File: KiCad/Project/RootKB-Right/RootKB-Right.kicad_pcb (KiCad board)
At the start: 2 copper layers, 137.4 x 107.4 mm, 69 parts, among them J1 OLED-128x32, U1 Arduino_Pro_Micro, U2 TRRS

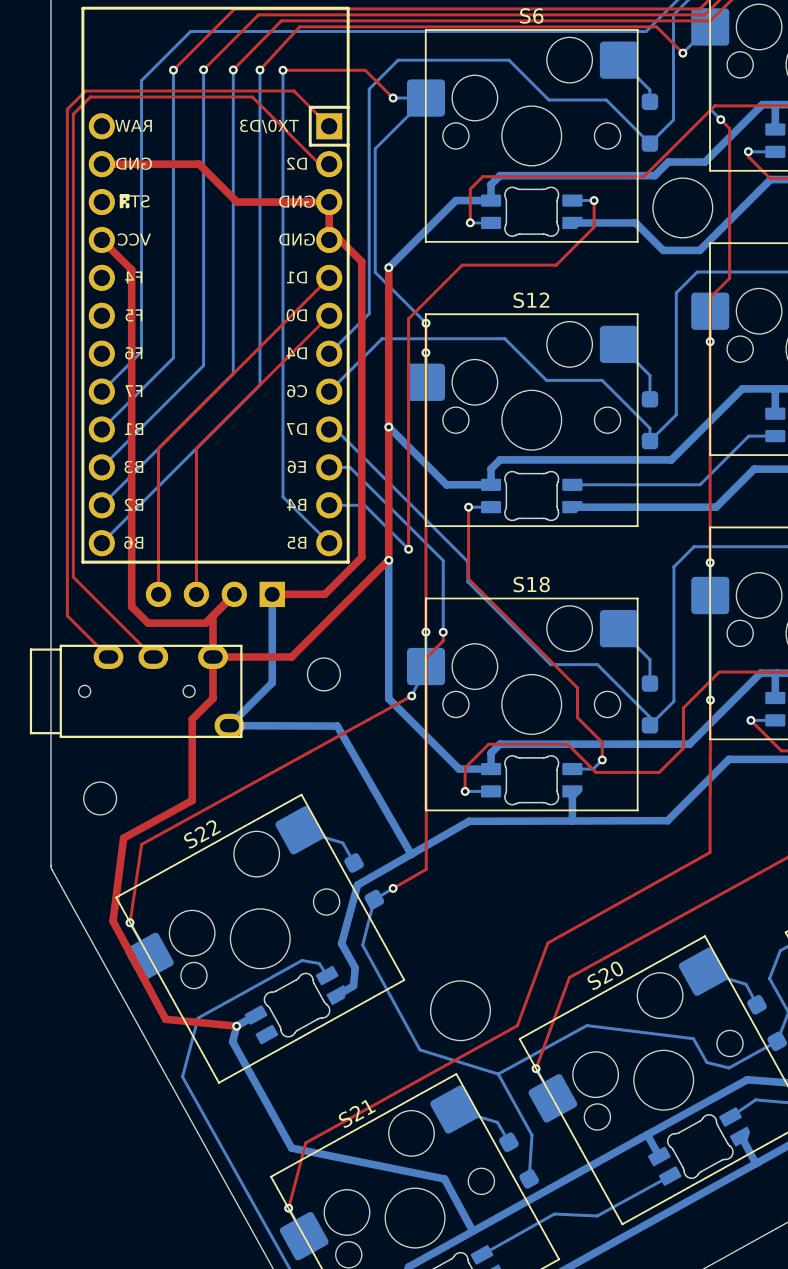
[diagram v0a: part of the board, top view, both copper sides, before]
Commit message: last updates
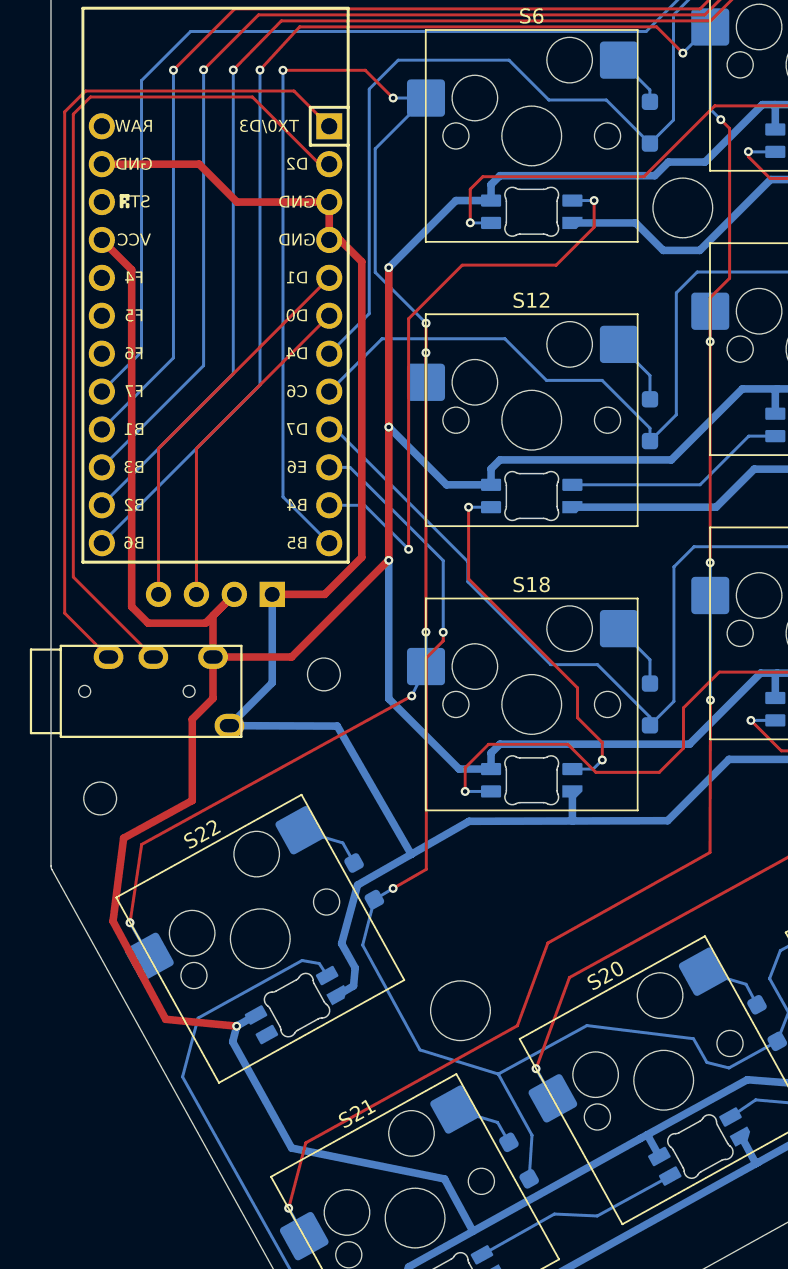
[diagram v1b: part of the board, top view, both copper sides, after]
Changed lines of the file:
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@@
 	(title_block
 		(title "RootKB-Right PCB")
-		(date "2024-05-05")
+		(date "2024-05-08")
 		(rev "1.0")
 	)
@@
 		(fp_arc
 			(start 1.749484 0.919721)
-			(mid 1.712534 0.814067)
+			(mid 1.71254 0.814067)
 			(end 1.699999 0.702843)
 			(stroke
@@
 		(fp_arc
 			(start -1.046711 1.568299)
-			(mid -1.63807 1.504035)
+			(mid -1.638071 1.504035)
 			(end -1.749484 0.919721)
 			(stroke
@@
 		(fp_arc
 			(start 1.749484 0.919721)
-			(mid 1.712534 0.814067)
+			(mid 1.712541 0.814066)
 			(end 1.7 0.702843)
 			(stroke
@@
 		(fp_arc
 			(start 0.794453 1.500001)
-			(mid 0.925123 1.517379)
+			(mid 0.925123 1.51738)
 			(end 1.046711 1.5683)
 			(stroke
@@
 		(fp_arc
 			(start 1.046711 -1.568296)
-			(mid 1.638069 -1.504033)
+			(mid 1.638074 -1.504031)
 			(end 1.749485 -0.919717)
 			(stroke
@@
 		(fp_arc
 			(start 1.04671 -1.568298)
-			(mid 0.925122 -1.517374)
+			(mid 0.925123 -1.517374)
 			(end 0.794452 -1.5)
 			(stroke
@@
 		(fp_arc
 			(start 1.749484 0.919721)
-			(mid 1.712534 0.814067)
+			(mid 1.71254 0.814067)
 			(end 1.699999 0.702843)
 			(stroke
@@
 		(fp_arc
 			(start -1.046711 1.568299)
-			(mid -1.63807 1.504035)
+			(mid -1.638071 1.504035)
 			(end -1.749484 0.919721)
 			(stroke
@@
 		(fp_arc
 			(start 1.749484 0.919721)
-			(mid 1.712534 0.814067)
+			(mid 1.712541 0.814066)
 			(end 1.7 0.702843)
 			(stroke
@@
 		(fp_arc
 			(start 0.794453 1.500001)
-			(mid 0.925123 1.517379)
+			(mid 0.925123 1.51738)
 			(end 1.046711 1.5683)
 			(stroke
@@
 		(fp_arc
 			(start 1.046711 -1.568296)
-			(mid 1.638069 -1.504033)
+			(mid 1.638074 -1.504031)
 			(end 1.749485 -0.919717)
 			(stroke
@@
 		(fp_arc
 			(start 1.04671 -1.568298)
-			(mid 0.925122 -1.517374)
+			(mid 0.925123 -1.517374)
 			(end 0.794452 -1.5)
 			(stroke
@@
 		(fp_arc
 			(start 1.749484 0.919721)
-			(mid 1.712534 0.814067)
+			(mid 1.71254 0.814067)
 			(end 1.699999 0.702843)
 			(stroke
@@
 		(fp_arc
 			(start -1.046711 1.568299)
-			(mid -1.63807 1.504035)
+			(mid -1.638071 1.504035)
 			(end -1.749484 0.919721)
 			(stroke
@@
 		(fp_arc
 			(start 1.749484 0.919721)
-			(mid 1.712534 0.814067)
+			(mid 1.71254 0.814067)
 			(end 1.699999 0.702843)
 			(stroke
@@
 		(fp_arc
 			(start -1.046711 1.568299)
-			(mid -1.63807 1.504035)
+			(mid -1.638071 1.504035)
 			(end -1.749484 0.919721)
 			(stroke
@@
 		(fp_arc
 			(start 1.749484 0.919721)
-			(mid 1.712534 0.814067)
+			(mid 1.71254 0.814067)
 			(end 1.699999 0.702843)
 			(stroke
@@
 		(fp_arc
 			(start -1.046711 1.568299)
-			(mid -1.63807 1.504035)
+			(mid -1.638071 1.504035)
 			(end -1.749484 0.919721)
 			(stroke
@@
 		(fp_arc
 			(start 1.749484 0.919721)
-			(mid 1.712534 0.814067)
+			(mid 1.71254 0.814067)
 			(end 1.699999 0.702843)
 			(stroke
@@
 		(fp_arc
 			(start -1.046711 1.568299)
-			(mid -1.63807 1.504035)
+			(mid -1.638071 1.504035)
 			(end -1.749484 0.919721)
 			(stroke
@@
 		(fp_arc
 			(start 1.749484 0.919721)
-			(mid 1.712534 0.814067)
+			(mid 1.71254 0.814067)
 			(end 1.699999 0.702843)
 			(stroke
@@
 		(fp_arc
 			(start -1.046711 1.568299)
-			(mid -1.63807 1.504035)
+			(mid -1.638071 1.504035)
 			(end -1.749484 0.919721)
 			(stroke
@@
 		(fp_arc
 			(start 1.749484 0.919721)
-			(mid 1.712534 0.814067)
+			(mid 1.712541 0.814066)
 			(end 1.7 0.702843)
 			(stroke
@@
 		(fp_arc
 			(start 0.794453 1.500001)
-			(mid 0.925123 1.517379)
+			(mid 0.925123 1.51738)
 			(end 1.046711 1.5683)
 			(stroke
@@
 		(fp_arc
 			(start 1.046711 -1.568296)
-			(mid 1.638069 -1.504033)
+			(mid 1.638074 -1.504031)
 			(end 1.749485 -0.919717)
 			(stroke
@@
 		(fp_arc
 			(start 1.04671 -1.568298)
-			(mid 0.925122 -1.517374)
+			(mid 0.925123 -1.517374)
 			(end 0.794452 -1.5)
 			(stroke
@@
 		(fp_arc
 			(start 1.749484 0.919721)
-			(mid 1.712534 0.814067)
+			(mid 1.71254 0.814067)
 			(end 1.699999 0.702843)
 			(stroke
@@
 		(fp_arc
 			(start -1.046711 1.568299)
-			(mid -1.63807 1.504035)
+			(mid -1.638071 1.504035)
 			(end -1.749484 0.919721)
 			(stroke
@@
 		(fp_arc
 			(start 1.749484 0.919721)
-			(mid 1.712534 0.814067)
+			(mid 1.71254 0.814067)
 			(end 1.699999 0.702843)
 			(stroke
@@
 		(fp_arc
 			(start -1.046711 1.568299)
-			(mid -1.63807 1.504035)
+			(mid -1.638071 1.504035)
 			(end -1.749484 0.919721)
 			(stroke
@@
 		(fp_arc
 			(start 1.749484 0.919721)
-			(mid 1.712534 0.814067)
+			(mid 1.71254 0.814067)
 			(end 1.699999 0.702843)
 			(stroke
@@
 		(fp_arc
 			(start -1.046711 1.568299)
-			(mid -1.63807 1.504035)
+			(mid -1.638071 1.504035)
 			(end -1.749484 0.919721)
 			(stroke
@@
 		(fp_arc
 			(start 1.749484 0.919721)
-			(mid 1.712534 0.814067)
+			(mid 1.71254 0.814067)
 			(end 1.699999 0.702843)
 			(stroke
@@
 		(fp_arc
 			(start -1.046711 1.568299)
-			(mid -1.63807 1.504035)
+			(mid -1.638071 1.504035)
 			(end -1.749484 0.919721)
 			(stroke
@@
 		(fp_arc
 			(start 1.749484 0.919721)
-			(mid 1.712534 0.814067)
+			(mid 1.71254 0.814067)
 			(end 1.699999 0.702843)
 			(stroke
@@
 		(fp_arc
 			(start -1.046711 1.568299)
-			(mid -1.63807 1.504035)
+			(mid -1.638071 1.504035)
 			(end -1.749484 0.919721)
 			(stroke
@@
 		(fp_arc
 			(start 1.749484 0.919721)
-			(mid 1.712534 0.814067)
+			(mid 1.71254 0.814067)
 			(end 1.699999 0.702843)
 			(stroke
@@
 		(fp_arc
 			(start -1.046711 1.568299)
-			(mid -1.63807 1.504035)
+			(mid -1.638071 1.504035)
 			(end -1.749484 0.919721)
 			(stroke
@@
 		(fp_arc
 			(start 1.749484 0.919721)
-			(mid 1.712534 0.814067)
+			(mid 1.71254 0.814067)
 			(end 1.699999 0.702843)
 			(stroke
@@
 		(fp_arc
 			(start -1.046711 1.568299)
-			(mid -1.63807 1.504035)
+			(mid -1.638071 1.504035)
 			(end -1.749484 0.919721)
 			(stroke
@@
 		(fp_arc
 			(start 1.749484 0.919721)
-			(mid 1.712534 0.814067)
+			(mid 1.71254 0.814067)
 			(end 1.699999 0.702843)
 			(stroke
@@
 		(fp_arc
 			(start -1.046711 1.568299)
-			(mid -1.63807 1.504035)
+			(mid -1.638071 1.504035)
 			(end -1.749484 0.919721)
 			(stroke
@@
 		(fp_arc
 			(start 1.749484 0.919721)
-			(mid 1.712534 0.814067)
+			(mid 1.712541 0.814066)
 			(end 1.7 0.702843)
 			(stroke
@@
 		(fp_arc
 			(start 0.794453 1.500001)
-			(mid 0.925123 1.517379)
+			(mid 0.925123 1.51738)
 			(end 1.046711 1.5683)
 			(stroke
@@
 		(fp_arc
 			(start 1.046711 -1.568296)
-			(mid 1.638069 -1.504033)
+			(mid 1.638074 -1.504031)
 			(end 1.749485 -0.919717)
 			(stroke
@@
 		(fp_arc
 			(start 1.04671 -1.568298)
-			(mid 0.925122 -1.517374)
+			(mid 0.925123 -1.517374)
 			(end 0.794452 -1.5)
 			(stroke
@@
 		(fp_arc
 			(start 1.749484 0.919721)
-			(mid 1.712534 0.814067)
+			(mid 1.71254 0.814067)
 			(end 1.699999 0.702843)
 			(stroke
@@
 		(fp_arc
 			(start -1.046711 1.568299)
-			(mid -1.63807 1.504035)
+			(mid -1.638071 1.504035)
 			(end -1.749484 0.919721)
 			(stroke
@@
 		(fp_arc
 			(start 1.749484 0.919721)
-			(mid 1.712534 0.814067)
+			(mid 1.71254 0.814067)
 			(end 1.699999 0.702843)
 			(stroke
@@
 		(fp_arc
 			(start -1.046711 1.568299)
-			(mid -1.63807 1.504035)
+			(mid -1.638071 1.504035)
 			(end -1.749484 0.919721)
 			(stroke
@@
 		(fp_arc
 			(start 1.749484 0.919721)
-			(mid 1.712534 0.814067)
+			(mid 1.71254 0.814067)
 			(end 1.699999 0.702843)
 			(stroke
@@
 		(fp_arc
 			(start -1.046711 1.568299)
-			(mid -1.63807 1.504035)
+			(mid -1.638071 1.504035)
 			(end -1.749484 0.919721)
 			(stroke
@@
 	)
 	(segment
-		(start 85.822657 93.909451)
-		(end 83.061949 91.148743)
+		(start 84.281949 55.977407)
+		(end 98.250404 55.977407)
 		(width 0.2)
 		(layer "F.Cu")
@@
 	)
 	(segment
-		(start 83.061949 91.148743)
-		(end 83.061949 57.197407)
+		(start 82.881949 90.968743)
+		(end 82.881949 57.377407)
 		(width 0.2)
 		(layer "F.Cu")
@@
 	)
 	(segment
-		(start 83.061949 57.197407)
-		(end 84.281949 55.977407)
+		(start 85.822657 93.909451)
+		(end 82.881949 90.968743)
 		(width 0.2)
 		(layer "F.Cu")
@@
 	)
 	(segment
-		(start 84.281949 55.977407)
-		(end 98.250404 55.977407)
+		(start 82.881949 57.377407)
+		(end 84.281949 55.977407)
 		(width 0.2)
 		(layer "F.Cu")
